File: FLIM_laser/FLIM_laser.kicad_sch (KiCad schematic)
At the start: 12 parts

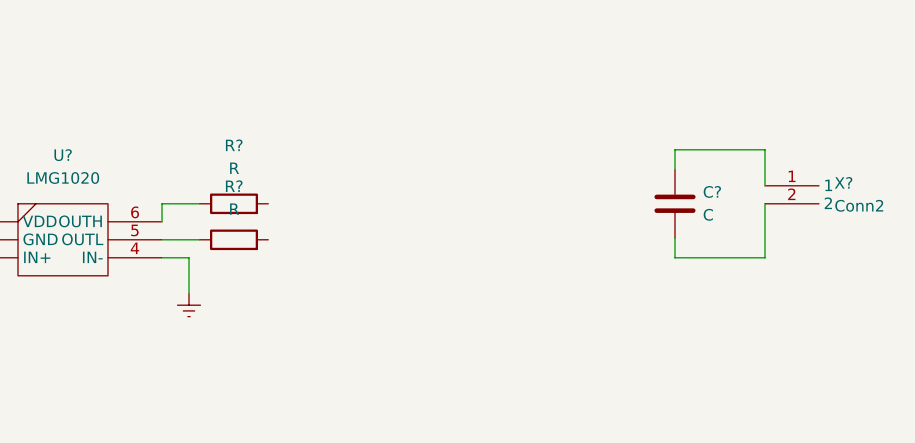
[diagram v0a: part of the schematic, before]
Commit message: v0.3 circuit is ready
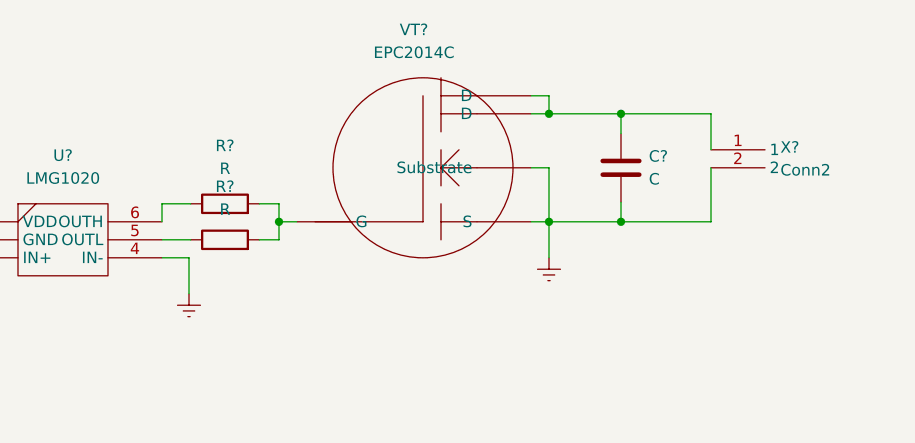
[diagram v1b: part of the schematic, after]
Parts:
- added VT?: EPC2014C, symbol FLIM_LASR:EPC2014C
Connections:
- net Earth: now also C?.2, X?.2, VT?. (Substrate)
- net at R?.2: now also R?.2, VT?. (Substrate)
- net at C?.1, X?.1: now also VT?. (Substrate)
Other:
- moved on the sheet: C?, R?, X?
